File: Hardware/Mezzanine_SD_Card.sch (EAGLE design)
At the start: 11 parts, among them U1 USD-SOCKETNEW, U2 EDISON_CONNECTOR_FULLMOUNTING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, U3 EDISON_CONNECTOR_FULLHEADER

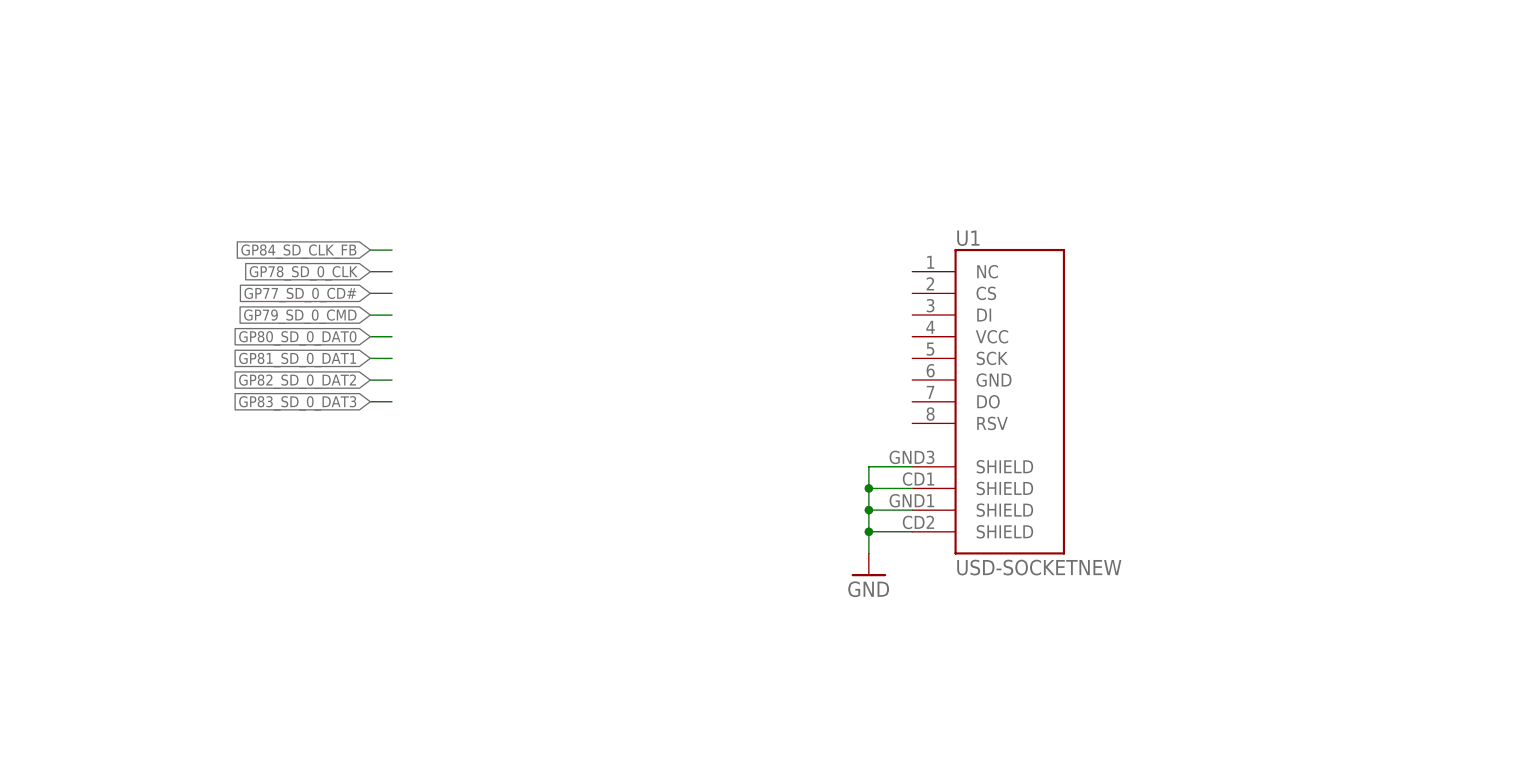
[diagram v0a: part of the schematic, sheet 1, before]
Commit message: Layout complete, Ready for review.
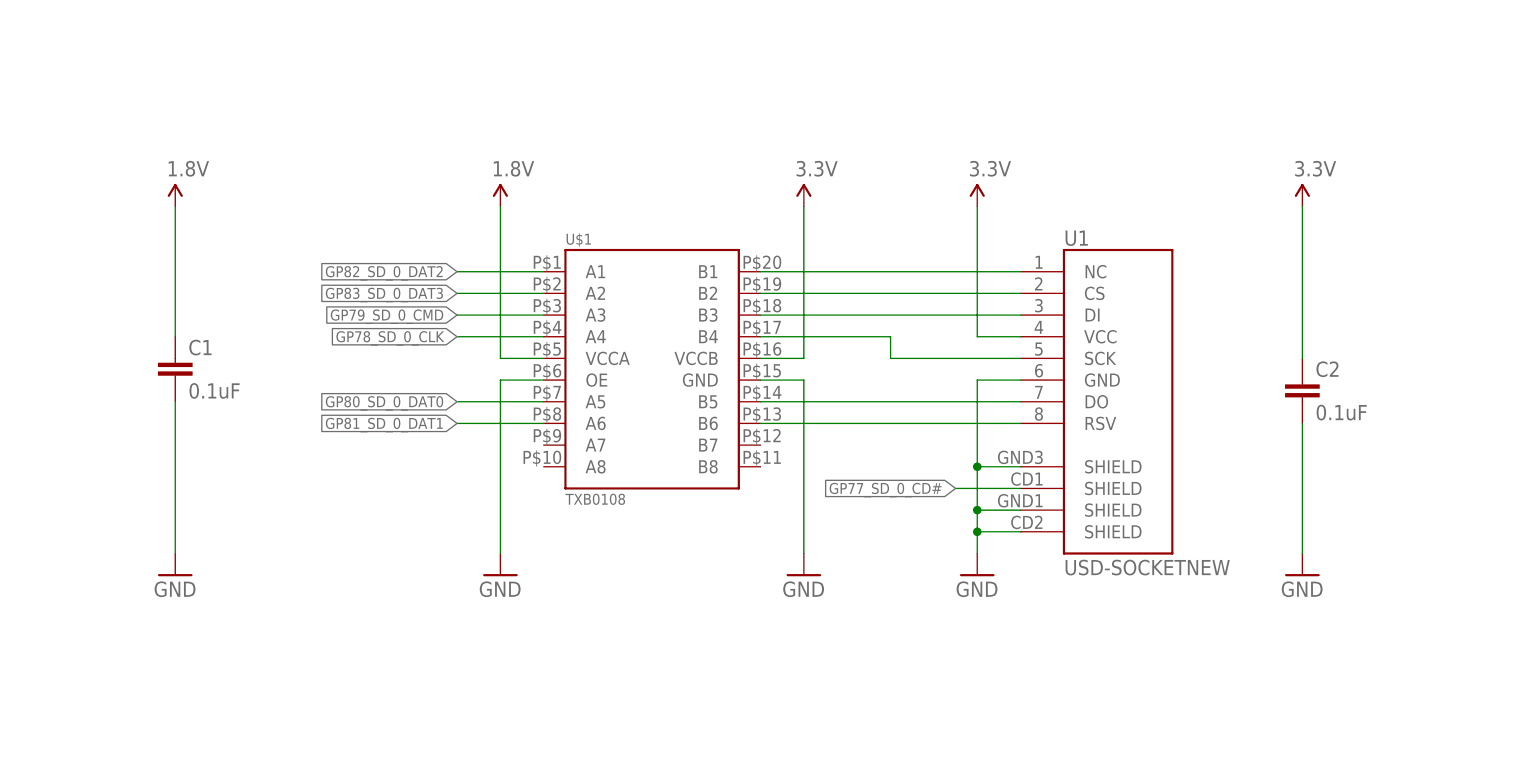
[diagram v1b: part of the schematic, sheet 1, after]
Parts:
- added C1, C2: 0.1uF, SparkFun-Capacitors:0.1UF-25V(+80/-20%)(0603)
- added U$1: TXB0108, Testing:TXB0108
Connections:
- new net N$1: U$1.B1, U1.NC
- new net N$2: U$1.B2, U1.CS
- new net N$3: U$1.B3, U1.DI
- new net N$4: U$1.B4, U1.SCK
- new net N$5: U$1.B5, U1.DO
- new net N$6: U$1.B6, U1.RSV
- net 1.8V: now also C1.1, U$1.VCCA
- net 3.3V: now also C2.1, U$1.VCCB, U1.VCC
- net GND: now also C1.2, C2.2, U$1.GND, U$1.OE, U1.GND; no longer U1.SHIELD@2
- net GP77_SD_0_CD#: now also U1.SHIELD@2
- net GP78_SD_0_CLK: now also U$1.A4
- net GP79_SD_0_CMD: now also U$1.A3
- net GP80_SD_0_DAT0: now also U$1.A5
- net GP81_SD_0_DAT1: now also U$1.A6
- net GP82_SD_0_DAT2: now also U$1.A1
- net GP83_SD_0_DAT3: now also U$1.A2
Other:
- moved on the sheet: U1
